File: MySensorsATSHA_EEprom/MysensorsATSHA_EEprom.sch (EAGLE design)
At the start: 3 parts, among them IC1 AT25DF512C-SSHN-B

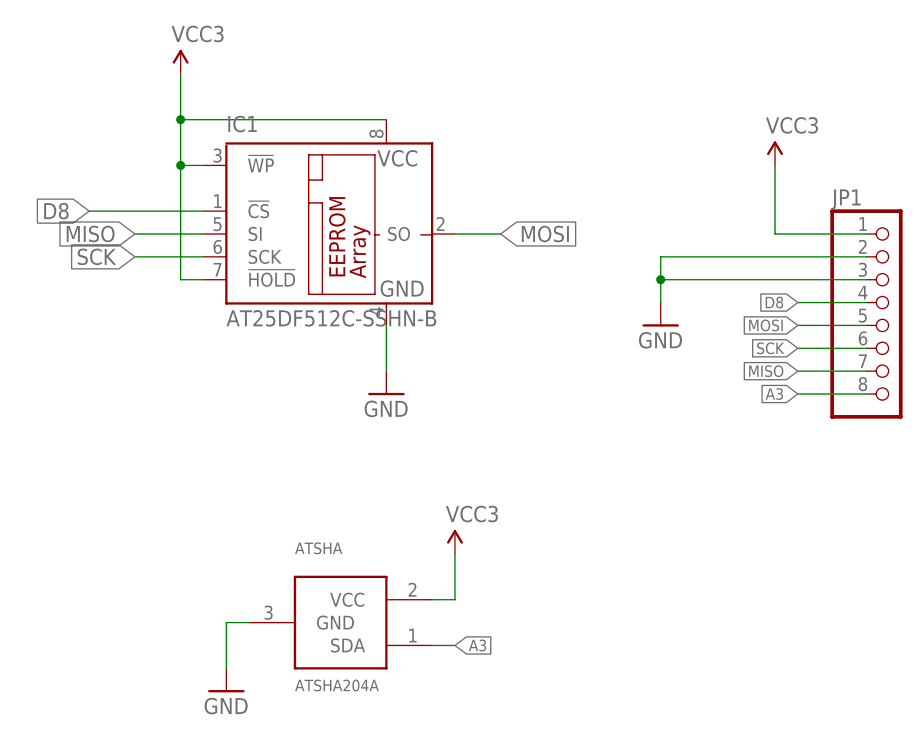
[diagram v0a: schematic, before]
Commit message: routing minor changes
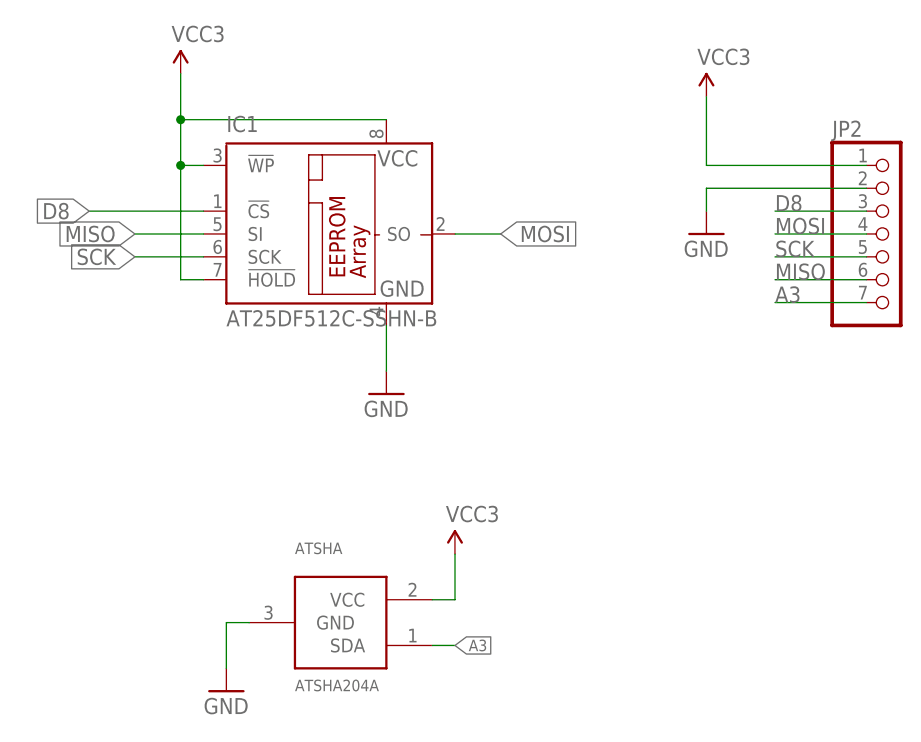
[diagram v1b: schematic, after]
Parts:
- removed JP1: (no value), adafruit:PINHD-1X8CLEANBIG
- added JP2: (no value), pinhead:PINHD-1X7
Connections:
- net A3: now also JP2.7; no longer JP1.8
- net D8: now also JP2.3; no longer JP1.4
- net GND: now also JP2.2; no longer JP1.2, JP1.3
- net MISO: now also JP2.6; no longer JP1.7
- net MOSI: now also JP2.4; no longer JP1.5
- net SCK: now also JP2.5; no longer JP1.6
- net VCC: now also JP2.1; no longer JP1.1
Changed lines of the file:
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@@
 <part name="VCC8" library="SparkFun-Aesthetics" deviceset="VCC" device="" value="VCC3"/>
 <part name="GND5" library="SparkFun-Aesthetics" deviceset="GND" device=""/>
-<part name="JP1" library="adafruit" deviceset="PINHD-1X8" device="CLEANBIG"/>
-<part name="GND1" library="SparkFun-Aesthetics" deviceset="GND" device=""/>
-<part name="VCC1" library="SparkFun-Aesthetics" deviceset="VCC" device="" value="VCC3"/>
+<part name="JP2" library="pinhead" deviceset="PINHD-1X7" device=""/>
+<part name="GND2" library="SparkFun-Aesthetics" deviceset="GND" device=""/>
+<part name="VCC2" library="SparkFun-Aesthetics" deviceset="VCC" device="" value="VCC3"/>
 </parts>
 <sheets>
@@
 <instance part="VCC8" gate="G$1" x="35.56" y="50.8"/>
 <instance part="GND5" gate="1" x="58.42" y="15.24"/>
-<instance part="JP1" gate="G$1" x="114.3" y="25.4"/>
-<instance part="GND1" gate="1" x="88.9" y="22.86"/>
-<instance part="VCC1" gate="G$1" x="101.6" y="40.64"/>
+<instance part="JP2" gate="A" x="114.3" y="33.02"/>
+<instance part="GND2" gate="1" x="93.98" y="33.02"/>
+<instance part="VCC2" gate="G$1" x="93.98" y="48.26"/>
 </instances>
 <busses>
@@
 </segment>
 <segment>
-<pinref part="JP1" gate="G$1" pin="1"/>
-<pinref part="VCC1" gate="G$1" pin="VCC"/>
-<wire x1="111.76" y1="33.02" x2="101.6" y2="33.02" width="0.1524" layer="91"/>
-<wire x1="101.6" y1="33.02" x2="101.6" y2="40.64" width="0.1524" layer="91"/>
+<pinref part="JP2" gate="A" pin="1"/>
+<pinref part="VCC2" gate="G$1" pin="VCC"/>
+<wire x1="111.76" y1="40.64" x2="93.98" y2="40.64" width="0.1524" layer="91"/>
+<wire x1="93.98" y1="40.64" x2="93.98" y2="48.26" width="0.1524" layer="91"/>
 </segment>
 </net>
@@
 </segment>
 <segment>
-<pinref part="JP1" gate="G$1" pin="3"/>
-<pinref part="GND1" gate="1" pin="GND"/>
-<wire x1="111.76" y1="27.94" x2="88.9" y2="27.94" width="0.1524" layer="91"/>
-<wire x1="88.9" y1="27.94" x2="88.9" y2="25.4" width="0.1524" layer="91"/>
-<pinref part="JP1" gate="G$1" pin="2"/>
-<wire x1="111.76" y1="30.48" x2="88.9" y2="30.48" width="0.1524" layer="91"/>
-<wire x1="88.9" y1="30.48" x2="88.9" y2="27.94" width="0.1524" layer="91"/>
-<junction x="88.9" y="27.94"/>
+<pinref part="JP2" gate="A" pin="2"/>
+<pinref part="GND2" gate="1" pin="GND"/>
+<wire x1="111.76" y1="38.1" x2="93.98" y2="38.1" width="0.1524" layer="91"/>
+<wire x1="93.98" y1="38.1" x2="93.98" y2="35.56" width="0.1524" layer="91"/>
 </segment>
 </net>
@@
 </segment>
 <segment>
-<pinref part="JP1" gate="G$1" pin="6"/>
-<wire x1="111.76" y1="20.32" x2="104.14" y2="20.32" width="0.1524" layer="91"/>
-<label x="104.14" y="20.32" size="1.27" layer="95" rot="R180" xref="yes"/>
+<pinref part="JP2" gate="A" pin="5"/>
+<wire x1="111.76" y1="30.48" x2="101.6" y2="30.48" width="0.1524" layer="91"/>
+<label x="101.6" y="30.48" size="1.778" layer="95"/>
 </segment>
 </net>
@@
 </segment>
 <segment>
-<pinref part="JP1" gate="G$1" pin="7"/>
-<wire x1="111.76" y1="17.78" x2="104.14" y2="17.78" width="0.1524" layer="91"/>
-<label x="104.14" y="17.78" size="1.27" layer="95" rot="R180" xref="yes"/>
+<pinref part="JP2" gate="A" pin="6"/>
+<wire x1="111.76" y1="27.94" x2="101.6" y2="27.94" width="0.1524" layer="91"/>
+<label x="101.6" y="27.94" size="1.778" layer="95"/>
 </segment>
 </net>
@@
 </segment>
 <segment>
-<pinref part="JP1" gate="G$1" pin="5"/>
-<wire x1="111.76" y1="22.86" x2="104.14" y2="22.86" width="0.1524" layer="91"/>
-<label x="104.14" y="22.86" size="1.27" layer="95" rot="R180" xref="yes"/>
+<pinref part="JP2" gate="A" pin="4"/>
+<wire x1="111.76" y1="33.02" x2="101.6" y2="33.02" width="0.1524" layer="91"/>
+<label x="101.6" y="33.02" size="1.778" layer="95"/>
 </segment>
 </net>
@@
 </segment>
 <segment>
-<pinref part="JP1" gate="G$1" pin="8"/>
-<wire x1="111.76" y1="15.24" x2="104.14" y2="15.24" width="0.1524" layer="91"/>
-<label x="104.14" y="15.24" size="1.27" layer="95" rot="R180" xref="yes"/>
+<pinref part="JP2" gate="A" pin="7"/>
+<wire x1="111.76" y1="25.4" x2="101.6" y2="25.4" width="0.1524" layer="91"/>
+<label x="101.6" y="25.4" size="1.778" layer="95"/>
 </segment>
 </net>
@@
 </segment>
 <segment>
-<pinref part="JP1" gate="G$1" pin="4"/>
-<wire x1="111.76" y1="25.4" x2="104.14" y2="25.4" width="0.1524" layer="91"/>
-<label x="104.14" y="25.4" size="1.27" layer="95" rot="R180" xref="yes"/>
+<pinref part="JP2" gate="A" pin="3"/>
+<wire x1="111.76" y1="35.56" x2="101.6" y2="35.56" width="0.1524" layer="91"/>
+<label x="101.6" y="35.56" size="1.778" layer="95"/>
 </segment>
 </net>
